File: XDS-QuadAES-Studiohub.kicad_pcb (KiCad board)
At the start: 2 copper layers, 34.2 x 45.3 mm, 4 parts, among them J1 WeurthRJ45-8p8c-2x2-615032243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, J2 DB9_Male_MountingHoles

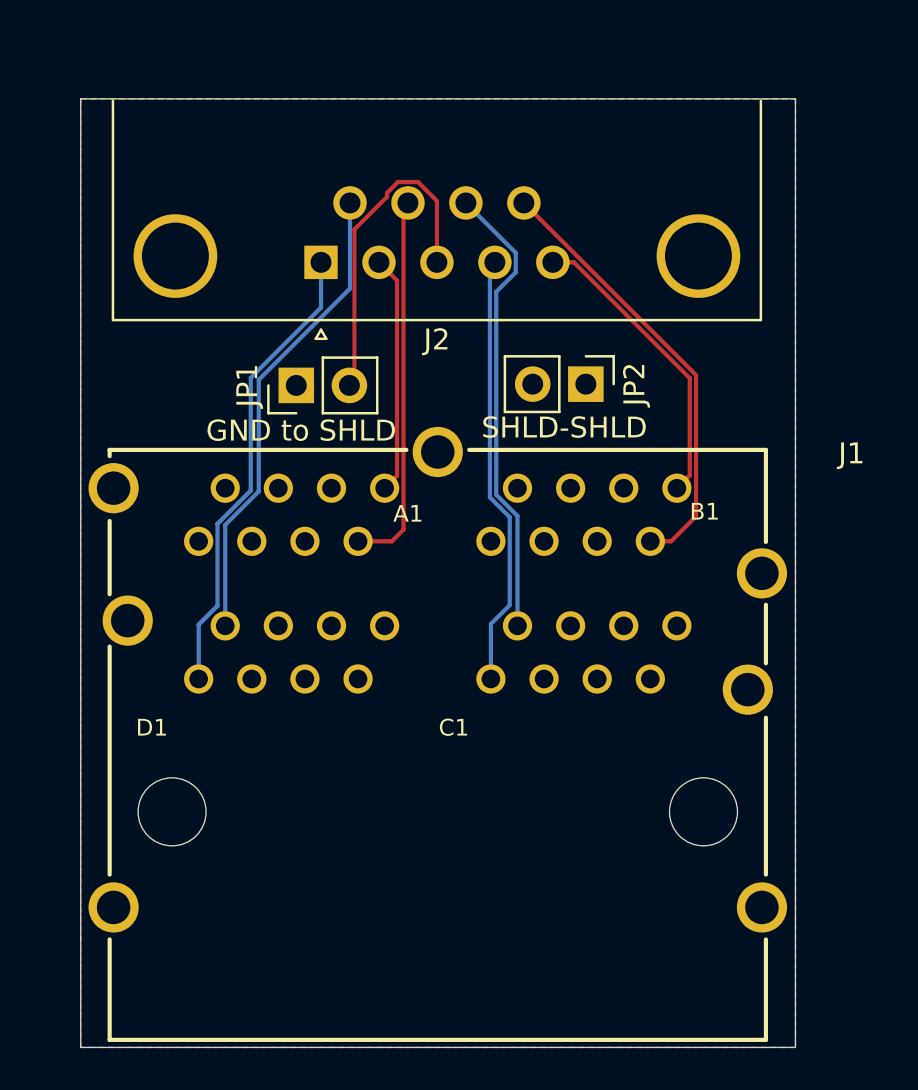
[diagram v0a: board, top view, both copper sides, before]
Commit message: minor changes
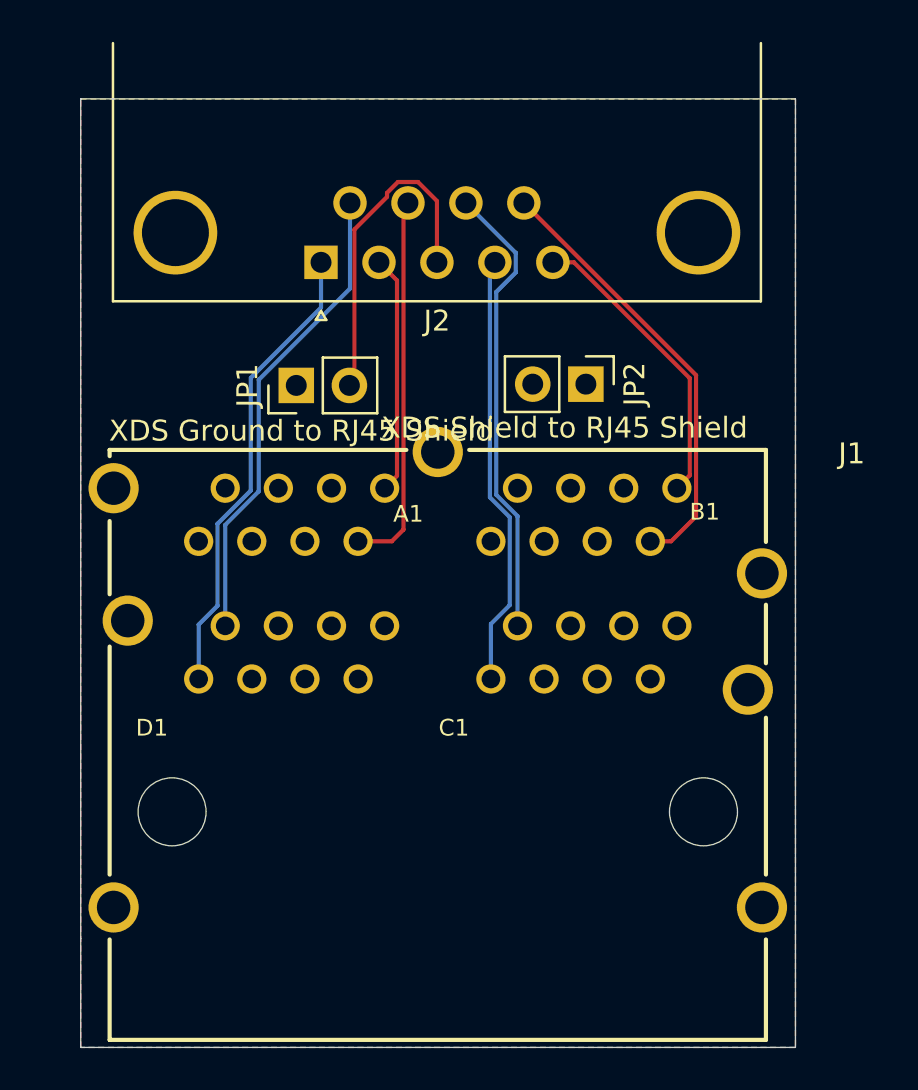
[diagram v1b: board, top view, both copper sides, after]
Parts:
- J1: footprint 615032243321 -> kicad:615032243321
- J2: value DB9_Male_MountingHoles -> DB9_Female; footprint Connector_Dsub:DSUB-9_Female_Horizontal_P2.77x2.84mm_EdgePinOffset4.94mm_Housed_MountingHolesOffset7.48mm -> Connector_Dsub:DSUB-9_Female_Horizontal_P2.77x2.84mm_EdgePinOffset7.70mm_Housed_MountingHolesOffset9.12mm
- JP1: value GND to SHLD -> XDS Ground to RJ45 Shield
- JP2: value SHLD-SHLD -> XDS Shield to RJ45 Shield
